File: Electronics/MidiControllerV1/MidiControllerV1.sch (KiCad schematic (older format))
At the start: 18 parts, among them J1 USB_B_Micro, J2 KeypadConnector, J3 OledConnector, J4 BluePillHeaderA, J5 BluepillHeaderB, SW1 Rotary_Encoder_Switch, SW2 Rotary_Encoder_Switch

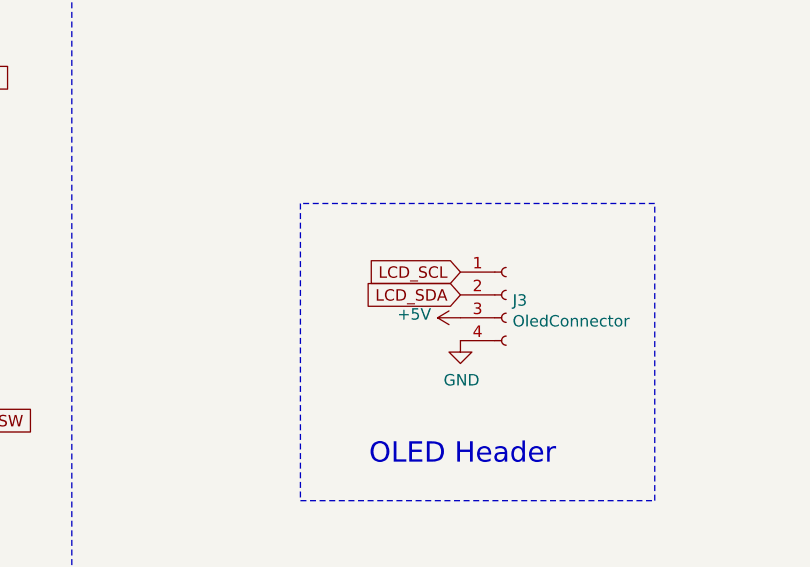
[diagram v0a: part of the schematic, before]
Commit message: #32 Updated pcb v1
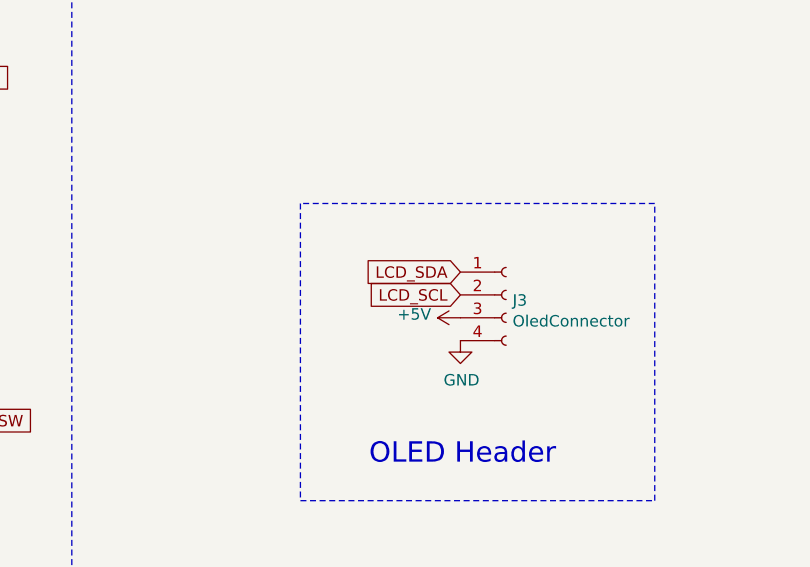
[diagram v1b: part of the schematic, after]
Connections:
- net LCD_SCL: now also J3.2 (Pin_2); no longer J3.1 (Pin_1)
- net LCD_SDA: now also J3.1 (Pin_1); no longer J3.2 (Pin_2)
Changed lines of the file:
@@
 	0    -1   -1   0
 $EndComp
+Text GLabel 5850 4850 0    50   Input ~ 0
+LCD_SDA
 Text GLabel 5850 4950 0    50   Input ~ 0
-LCD_SDA
-Text GLabel 5850 4850 0    50   Input ~ 0
 LCD_SCL
 Text GLabel 8600 3900 0    50   Input ~ 0
